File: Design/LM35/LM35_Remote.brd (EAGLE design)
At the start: 14.9 x 67.3 mm, 6 parts

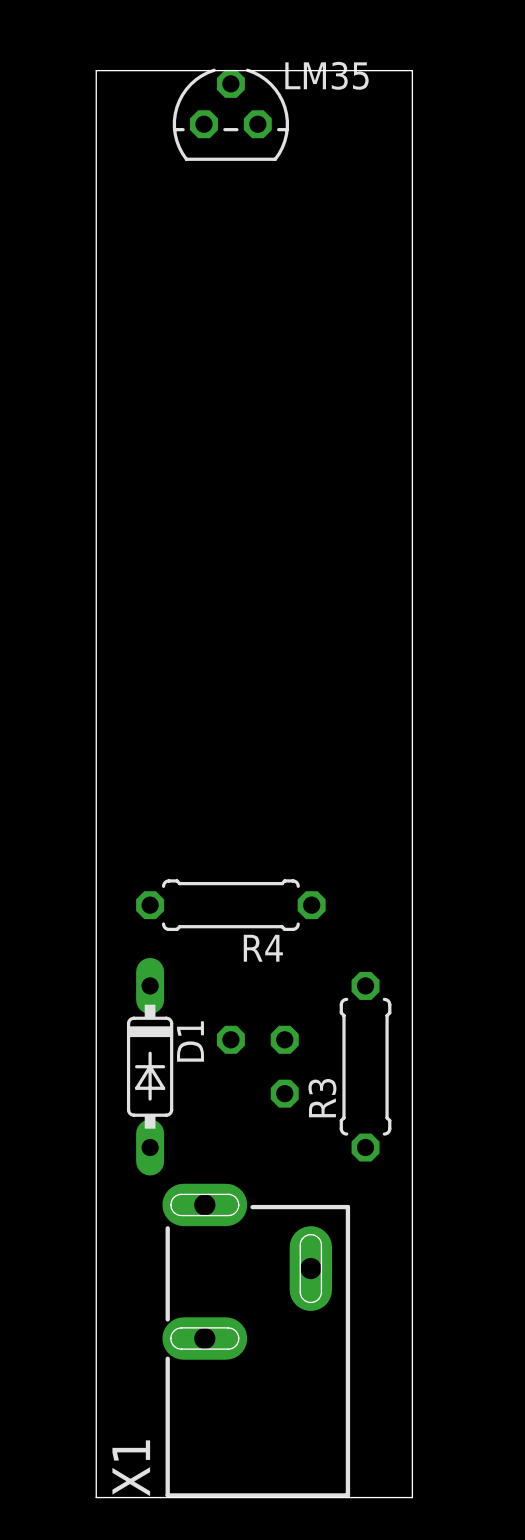
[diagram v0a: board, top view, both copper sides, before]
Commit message: Ultima revision del resumen semanal
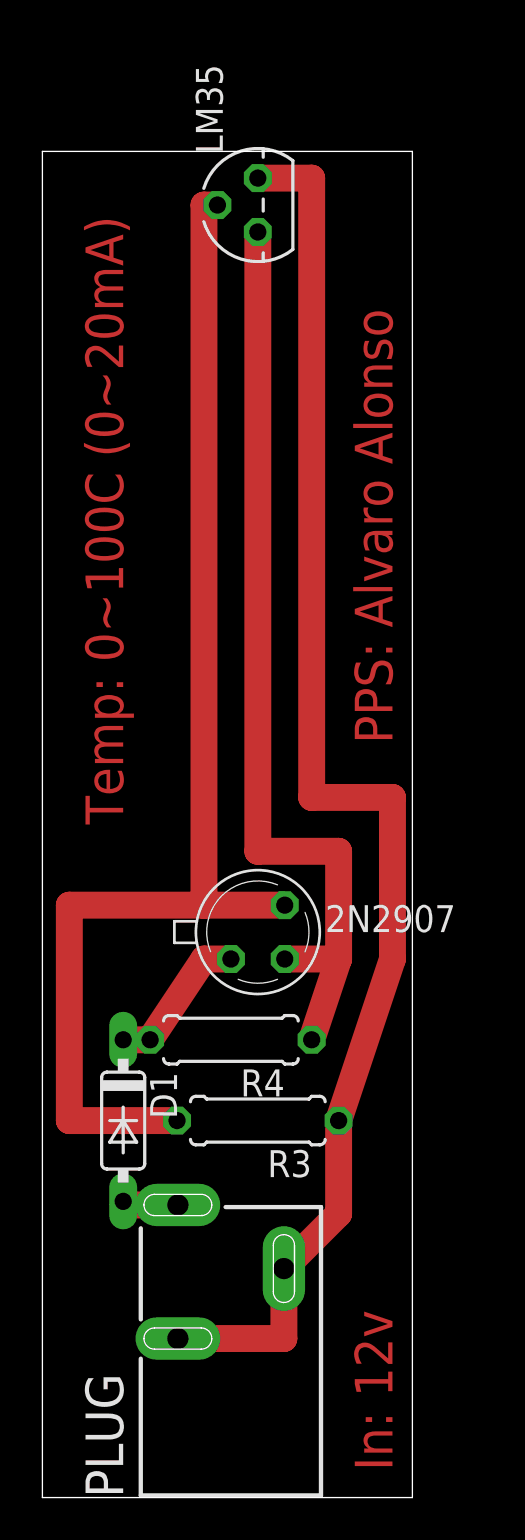
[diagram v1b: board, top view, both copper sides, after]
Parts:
- removed X1: (no value), con-shiua-chyuan:SCD-014-A
- added PLUG: (no value), con-shiua-chyuan:SCD-014-A
- moved 2N2907 6.35 mm to (95.2, 26.7), flipped to the top, turned to 0 degrees
- moved R4 6.35 mm to (94.0, 21.6)
- moved R3 5.68 mm to (95.2, 17.8), turned to 180 degrees
- moved LM35 4.02 mm to (95.2, 61.0), turned to 90 degrees
- moved D1 2.84 mm to (88.9, 17.8)
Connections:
- net N$4: now also PLUG.2, PLUG.3; no longer X1.2, X1.3
- net N$5: now also PLUG.1; no longer X1.1
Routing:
- net N$4: track 0.00 -> 67.6 mm
- net N$2: track 0.00 -> 59.1 mm
- net N$1: track 0.00 -> 44.7 mm
- net N$3: track 0.00 -> 7.12 mm
- net N$5: track 0.00 -> 2.75 mm
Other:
- board size 14.9 x 67.3 mm -> 17.5 x 63.5 mm
- board text added: "In: 12v"
- board text added: "PPS: Alvaro Alonso"
- board text added: "Temp: 0~100C (0~20mA)"
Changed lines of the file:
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@@
 <board>
 <plain>
-<wire x1="87.63" y1="0" x2="102.54" y2="0" width="0" layer="20"/>
-<wire x1="102.54" y1="0" x2="102.54" y2="67.3" width="0" layer="20"/>
-<wire x1="102.54" y1="67.3" x2="87.63" y2="67.3" width="0" layer="20"/>
-<wire x1="87.63" y1="67.3" x2="87.63" y2="0" width="0" layer="20"/>
+<wire x1="85.09" y1="0" x2="102.54" y2="0" width="0" layer="20"/>
+<wire x1="102.54" y1="0" x2="102.54" y2="63.49" width="0" layer="20"/>
+<wire x1="102.54" y1="63.49" x2="85.09" y2="63.49" width="0" layer="20"/>
+<wire x1="85.09" y1="63.49" x2="85.09" y2="0" width="0" layer="20"/>
+<text x="88.9" y="31.75" size="1.778" layer="1" rot="R90">Temp: 0~100C (0~20mA)</text>
+<text x="101.6" y="1.27" size="1.778" layer="1" rot="R90">In: 12v</text>
+<text x="101.6" y="35.56" size="1.778" layer="1" rot="R90">PPS: Alvaro Alonso</text>
+<dimension x1="85.09" y1="63.49" x2="85.09" y2="0" x3="80.01" y3="31.745" textsize="1.778" layer="1"/>
+<dimension x1="102.54" y1="63.49" x2="85.09" y2="63.49" x3="93.815" y3="67.31" textsize="1.778" layer="1"/>
 </plain>
 <attributes>
@@
 <classes>
 <class number="0" name="default" width="0" drill="0">
+<clearance class="0" value="0.205"/>
 </class>
 </classes>
-<designrules name="default">
+<designrules name="default *">
 <description language="de">&lt;b&gt;EAGLE Design Rules&lt;/b&gt;
 &lt;p&gt;
-Die Standard-Design-Rules sind so gewählt, dass sie für
+Die Standard-Design-Rules sind so gewÃÂ¤hlt, dass sie fÃÂ¼r
 die meisten Anwendungen passen. Sollte ihre Platine
 besondere Anforderungen haben, treffen Sie die erforderlichen
@@
 <param name="mtCopper" value="0.035mm 0.035mm 0.035mm 0.035mm 0.035mm 0.035mm 0.035mm 0.035mm 0.035mm 0.035mm 0.035mm 0.035mm 0.035mm 0.035mm 0.035mm 0.035mm"/>
 <param name="mtIsolate" value="1.5mm 0.15mm 0.2mm 0.15mm 0.2mm 0.15mm 0.2mm 0.15mm 0.2mm 0.15mm 0.2mm 0.15mm 0.2mm 0.15mm 0.2mm"/>
-<param name="mdWireWire" value="8mil"/>
-<param name="mdWirePad" value="8mil"/>
-<param name="mdWireVia" value="8mil"/>
-<param name="mdPadPad" value="8mil"/>
-<param name="mdPadVia" value="8mil"/>
-<param name="mdViaVia" value="8mil"/>
+<param name="mdWireWire" value="20mil"/>
+<param name="mdWirePad" value="20mil"/>
+<param name="mdWireVia" value="20mil"/>
+<param name="mdPadPad" value="20mil"/>
+<param name="mdPadVia" value="20mil"/>
+<param name="mdViaVia" value="20mil"/>
 <param name="mdSmdPad" value="8mil"/>
 <param name="mdSmdVia" value="8mil"/>
@@
 <param name="mdDrill" value="8mil"/>
 <param name="mdSmdStop" value="0mil"/>
-<param name="msWidth" value="10mil"/>
-<param name="msDrill" value="24mil"/>
+<param name="msWidth" value="30mil"/>
+<param name="msDrill" value="35mil"/>
 <param name="msMicroVia" value="9.99mm"/>
 <param name="msBlindViaRatio" value="0.5"/>
@@
 <autorouter>
 <pass name="Default">
-<param name="RoutingGrid" value="50mil"/>
+<param name="RoutingGrid" value="12.5mil"/>
 <param name="AutoGrid" value="1"/>
 <param name="Efforts" value="0"/>
 <param name="TopRouterVariant" value="1"/>
 <param name="tpViaShape" value="round"/>
-<param name="PrefDir.1" value="a"/>
+<param name="PrefDir.1" value="-"/>
 <param name="PrefDir.2" value="0"/>
 <param name="PrefDir.3" value="0"/>
@@
 </autorouter>
 <elements>
-<element name="2N2907" library="transistor" package="TO18" value="" x="95.25" y="20.32" rot="MR180"/>
-<element name="D1" library="diode" package="DO35-7" value="1N4148DO35-7" x="90.17" y="20.32" rot="R270"/>
-<element name="R3" library="resistor" package="0207/7" value="50-0.5%" x="100.33" y="20.32" rot="R90">
-<attribute name="SPICEPREFIX" value="R" x="100.33" y="20.32" size="1.778" layer="27" rot="R90" display="off"/>
+<element name="2N2907" library="transistor" package="TO18" value="" x="95.25" y="26.67"/>
+<element name="D1" library="diode" package="DO35-7" value="1N4148DO35-7" x="88.9" y="17.78" rot="R270"/>
+<element name="R3" library="resistor" package="0207/7" value="50-0.5%" x="95.25" y="17.78" rot="R180">
+<attribute name="SPICEPREFIX" value="R" x="95.25" y="17.78" size="1.778" layer="27" rot="R180" display="off"/>
 </element>
-<element name="R4" library="resistor" package="0207/7" value="4.7K" x="93.98" y="27.94" rot="R180">
-<attribute name="SPICEPREFIX" value="R" x="93.98" y="27.94" size="1.778" layer="27" rot="R180" display="off"/>
+<element name="R4" library="resistor" package="0207/7" value="4.7K" x="93.98" y="21.59" rot="R180">
+<attribute name="SPICEPREFIX" value="R" x="93.98" y="21.59" size="1.778" layer="27" rot="R180" display="off"/>
 </element>
-<element name="LM35" library="lm35" package="TO92" value="LM35CZ" x="93.98" y="64.77"/>
-<element name="X1" library="con-shiua-chyuan" package="SCD-014-A" value="" x="95.25" y="0">
-<attribute name="OC_NEWARK" value="unknown" x="95.25" y="0" size="1.778" layer="27" display="off"/>
-<attribute name="MPN" value="" x="95.25" y="0" size="1.778" layer="27" display="off"/>
-<attribute name="MF" value="" x="95.25" y="0" size="1.778" layer="27" display="off"/>
-<attribute name="OC_FARNELL" value="unknown" x="95.25" y="0" size="1.778" layer="27" display="off"/>
+<element name="LM35" library="lm35" package="TO92" value="LM35CZ" x="95.25" y="60.96" rot="R90"/>
+<element name="PLUG" library="con-shiua-chyuan" package="SCD-014-A" value="" x="93.98" y="0">
+<attribute name="OC_NEWARK" value="unknown" x="93.98" y="0" size="1.778" layer="27" display="off"/>
+<attribute name="MPN" value="" x="93.98" y="0" size="1.778" layer="27" display="off"/>
+<attribute name="MF" value="" x="93.98" y="0" size="1.778" layer="27" display="off"/>
+<attribute name="OC_FARNELL" value="unknown" x="93.98" y="0" size="1.778" layer="27" display="off"/>
 </element>
 </elements>
@@
 <contactref element="2N2907" pad="2"/>
 <contactref element="LM35" pad="1"/>
-<wire x1="97.79" y1="27.94" x2="92.71" y2="64.77" width="0" layer="19" extent="1-1"/>
-<wire x1="96.52" y1="21.59" x2="97.79" y2="27.94" width="0" layer="19" extent="1-1"/>
+<wire x1="97.79" y1="21.59" x2="99.06" y2="25.4" width="1.27" layer="1"/>
+<wire x1="99.06" y1="25.4" x2="99.06" y2="30.48" width="1.27" layer="1"/>
+<wire x1="96.52" y1="25.4" x2="99.06" y2="25.4" width="1.27" layer="1"/>
+<wire x1="99.06" y1="30.48" x2="95.25" y2="30.48" width="1.27" layer="1"/>
+<wire x1="95.25" y1="30.48" x2="95.25" y2="59.69" width="1.27" layer="1"/>
 </signal>
 <signal name="N$2">
@@
 <contactref element="R3" pad="2"/>
 <contactref element="LM35" pad="2"/>
-<wire x1="96.52" y1="19.05" x2="93.98" y2="66.675" width="0" layer="19" extent="1-1"/>
-<wire x1="100.33" y1="24.13" x2="96.52" y2="19.05" width="0" layer="19" extent="1-1"/>
+<wire x1="91.44" y1="17.78" x2="86.36" y2="17.78" width="1.27" layer="1"/>
+<wire x1="86.36" y1="17.78" x2="86.36" y2="27.94" width="1.27" layer="1"/>
+<wire x1="96.52" y1="27.94" x2="92.71" y2="27.94" width="1.27" layer="1"/>
+<wire x1="86.36" y1="27.94" x2="92.71" y2="27.94" width="1.27" layer="1"/>
+<wire x1="92.71" y1="27.94" x2="92.71" y2="60.96" width="1.27" layer="1"/>
+<wire x1="92.71" y1="60.96" x2="93.345" y2="60.96" width="1.27" layer="1"/>
 </signal>
 <signal name="N$3">
@@
 <contactref element="D1" pad="C"/>
 <contactref element="2N2907" pad="1"/>
-<wire x1="93.98" y1="21.59" x2="90.17" y2="27.94" width="0" layer="19" extent="1-1"/>
-<wire x1="90.17" y1="24.13" x2="93.98" y2="21.59" width="0" layer="19" extent="1-1"/>
+<wire x1="88.9" y1="21.59" x2="90.17" y2="21.59" width="1.27" layer="1"/>
+<wire x1="90.17" y1="21.59" x2="92.71" y2="25.4" width="1.27" layer="1"/>
+<wire x1="92.71" y1="25.4" x2="93.98" y2="25.4" width="1.27" layer="1"/>
 </signal>
 <signal name="N$4">
 <contactref element="R3" pad="1"/>
 <contactref element="LM35" pad="3"/>
-<contactref element="X1" pad="2"/>
-<contactref element="X1" pad="3"/>
-<wire x1="100.33" y1="16.51" x2="95.25" y2="64.77" width="0" layer="19" extent="1-1"/>
-<wire x1="97.75" y1="10.8" x2="100.33" y2="16.51" width="0" layer="19" extent="1-1"/>
-<wire x1="92.75" y1="7.5" x2="97.75" y2="10.8" width="0" layer="19" extent="1-1"/>
+<contactref element="PLUG" pad="2"/>
+<contactref element="PLUG" pad="3"/>
+<wire x1="91.48" y1="7.5" x2="96.48" y2="7.5" width="1.27" layer="1"/>
+<wire x1="96.48" y1="7.5" x2="96.48" y2="10.8" width="1.27" layer="1"/>
+<wire x1="96.48" y1="10.8" x2="99.06" y2="13.38" width="1.27" layer="1"/>
+<wire x1="99.06" y1="13.38" x2="99.06" y2="17.78" width="1.27" layer="1"/>
+<wire x1="99.06" y1="17.78" x2="101.6" y2="25.4" width="1.27" layer="1"/>
+<wire x1="101.6" y1="25.4" x2="101.6" y2="33.02" width="1.27" layer="1"/>
+<wire x1="101.6" y1="33.02" x2="97.79" y2="33.02" width="1.27" layer="1"/>
+<wire x1="97.79" y1="33.02" x2="97.79" y2="62.23" width="1.27" layer="1"/>
+<wire x1="97.79" y1="62.23" x2="95.25" y2="62.23" width="1.27" layer="1"/>
 </signal>
 <signal name="N$5">
 <contactref element="D1" pad="A"/>
-<contactref element="X1" pad="1"/>
-<wire x1="92.75" y1="13.8" x2="90.17" y2="16.51" width="0" layer="19" extent="1-1"/>
+<contactref element="PLUG" pad="1"/>
+<wire x1="91.48" y1="13.8" x2="88.9" y2="13.8" width="1.27" layer="1"/>
+<wire x1="88.9" y1="13.8" x2="88.9" y2="13.97" width="1.27" layer="1"/>
 </signal>
 </signals>

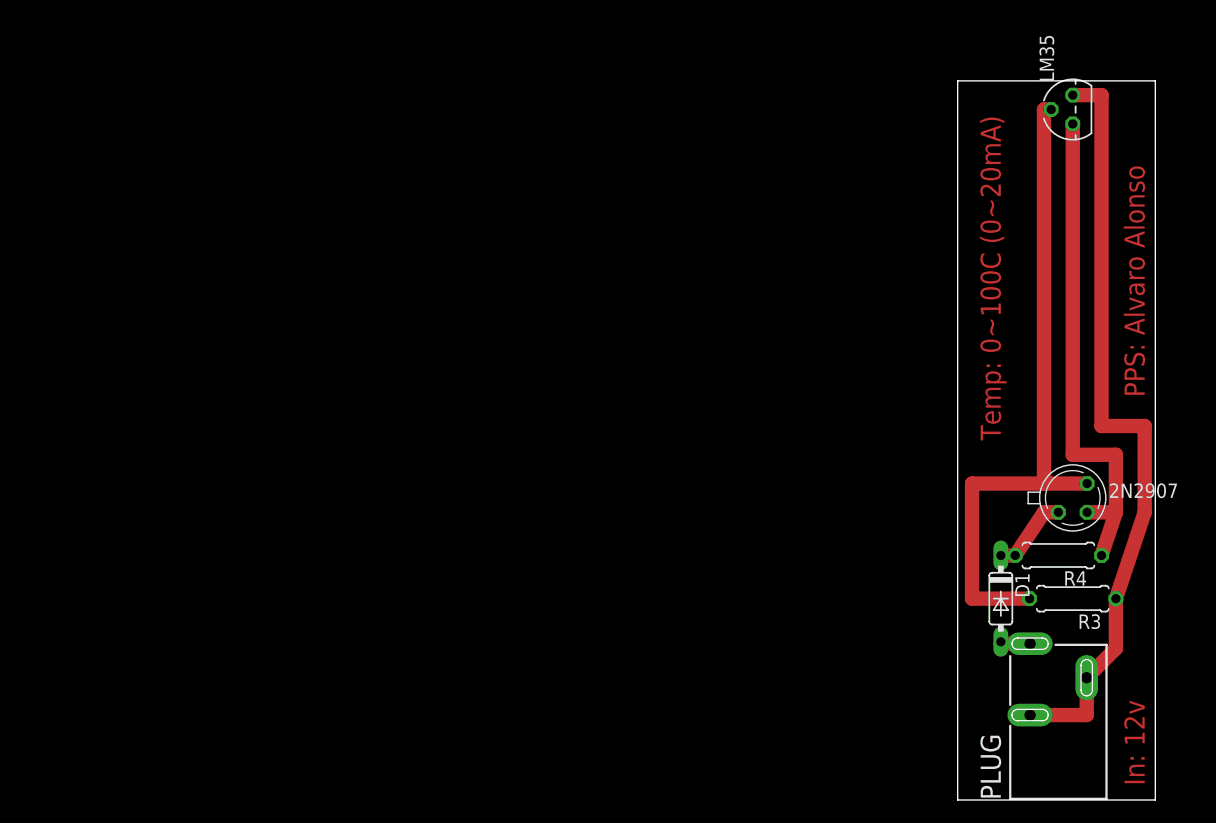
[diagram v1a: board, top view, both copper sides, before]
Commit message: Ultima modificacion plaqueta sensor
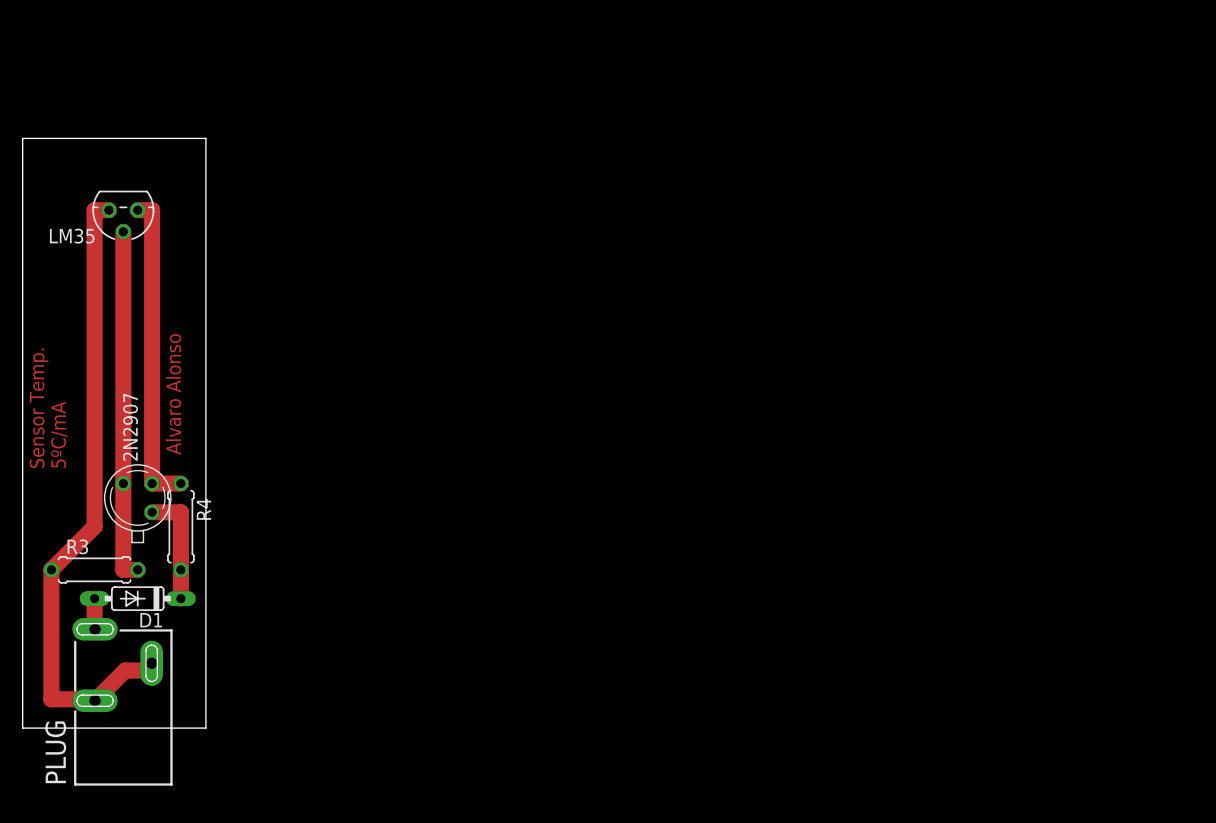
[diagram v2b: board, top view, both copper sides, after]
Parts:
- moved R3 86.4 mm to (8.89, 20.3), turned to 0 degrees
- moved LM35 84.3 mm to (11.4, 52.1), turned to 180 degrees
- moved PLUG 82.6 mm to (11.4, 1.27)
- moved 2N2907 82.5 mm to (12.7, 26.7), turned to 90 degrees
- moved R4 77.5 mm to (16.5, 24.1), turned to 270 degrees
- moved D1 76.2 mm to (12.7, 17.8), turned to 180 degrees
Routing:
- net N$2: track 59.1 -> 31.1 mm
- net N$1: track 44.7 -> 27.9 mm
- net N$4: track 67.6 -> 56.8 mm
- net N$3: track 7.12 -> 10.2 mm
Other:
- board size 17.5 x 63.5 mm -> 16.2 x 52.1 mm
- board text added: "Alvaro Alonso"
- board text added: "Sensor Temp. 5ºC/mA"
- board text removed: "In: 12v"
- board text removed: "PPS: Alvaro Alonso"
- board text removed: "Temp: 0~100C (0~20mA)"
